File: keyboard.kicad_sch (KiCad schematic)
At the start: 0 parts

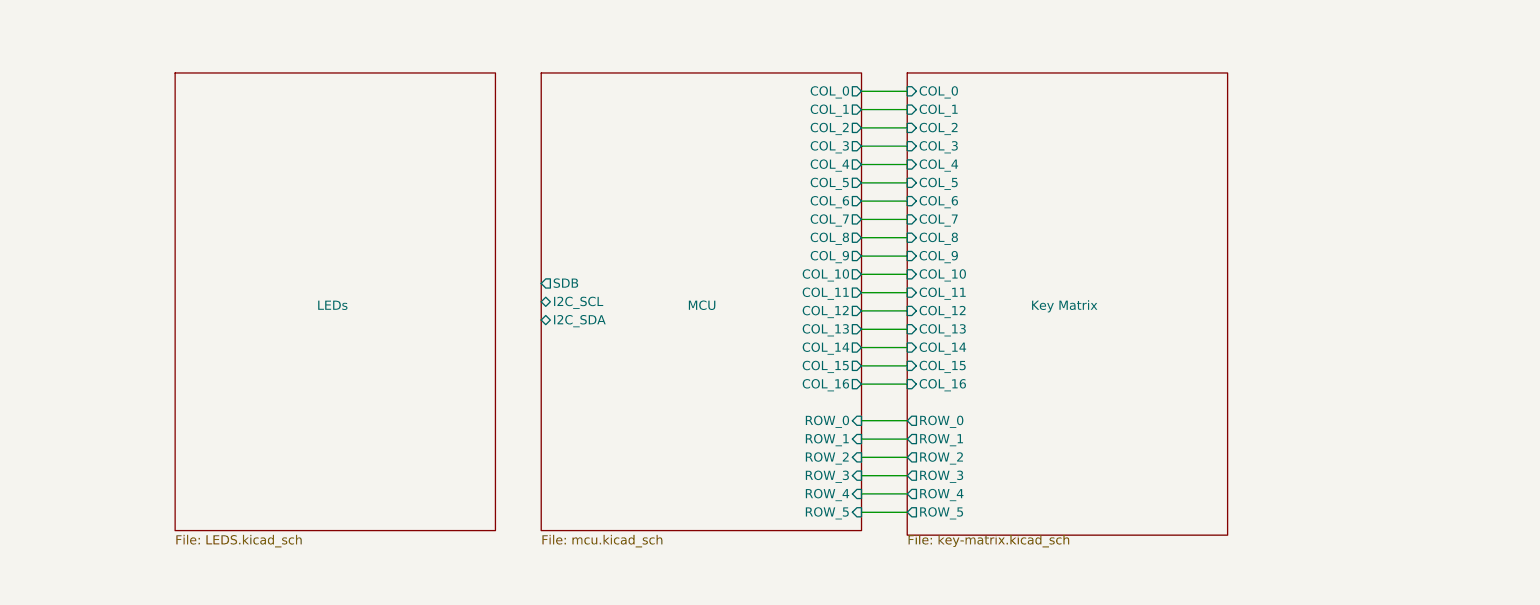
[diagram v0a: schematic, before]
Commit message: first draft
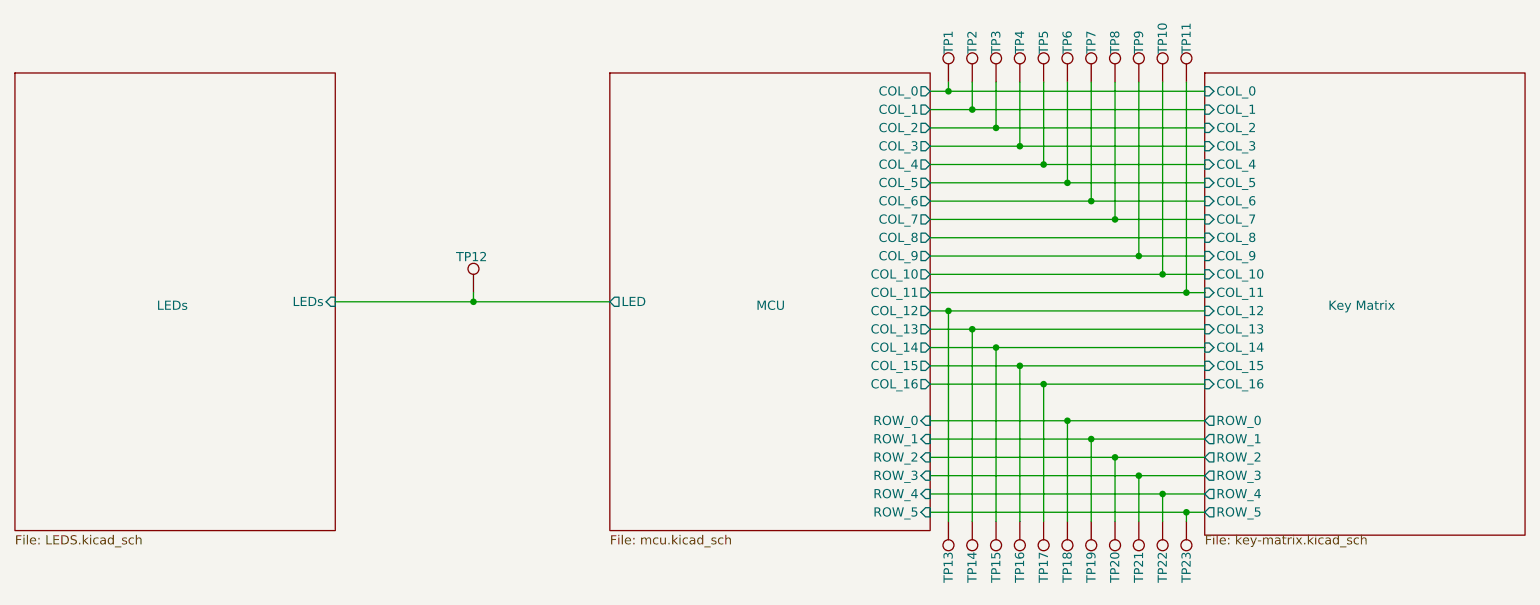
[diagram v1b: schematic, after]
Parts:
- added TP1, TP10, TP11, TP12, TP13, TP14, TP15, TP16, TP17, TP18, TP19, TP2, TP20, TP21, TP22, TP23, TP3, TP4, TP5, TP6, TP7, TP8, TP9: TestPoint, symbol Connector:TestPoint
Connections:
- net Key Matrix/COL_0: now also TP1.1
- net Key Matrix/COL_1: now also TP2.1
- net Key Matrix/COL_10: now also TP10.1
- net Key Matrix/COL_11: now also TP11.1
- net Key Matrix/COL_12: now also TP13.1
- net Key Matrix/COL_13: now also TP14.1
- net Key Matrix/COL_14: now also TP15.1
- net Key Matrix/COL_15: now also TP16.1
- net Key Matrix/COL_16: now also TP17.1
- net Key Matrix/COL_2: now also TP3.1
- net Key Matrix/COL_3: now also TP4.1
- net Key Matrix/COL_4: now also TP5.1
- net Key Matrix/COL_5: now also TP6.1
- net Key Matrix/COL_6: now also TP7.1
- net Key Matrix/COL_7: now also TP8.1
- net Key Matrix/COL_9: now also TP9.1
- net Key Matrix/ROW_0: now also TP18.1
- net Key Matrix/ROW_1: now also TP19.1
- net Key Matrix/ROW_2: now also TP20.1
- net Key Matrix/ROW_3: now also TP21.1
- net Key Matrix/ROW_4: now also TP22.1
- net Key Matrix/ROW_5: now also TP23.1
- new net LEDs/LEDs: TP12.1
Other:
- sheet LEDs ports: added LEDs; removed none
- sheet MCU ports: added LED; removed I2C_SCL, I2C_SDA, SDB
